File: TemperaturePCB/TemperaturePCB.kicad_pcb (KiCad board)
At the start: 2 copper layers, 16 x 24.8 mm, 3 parts, among them J1 Conn_01x02_Socket

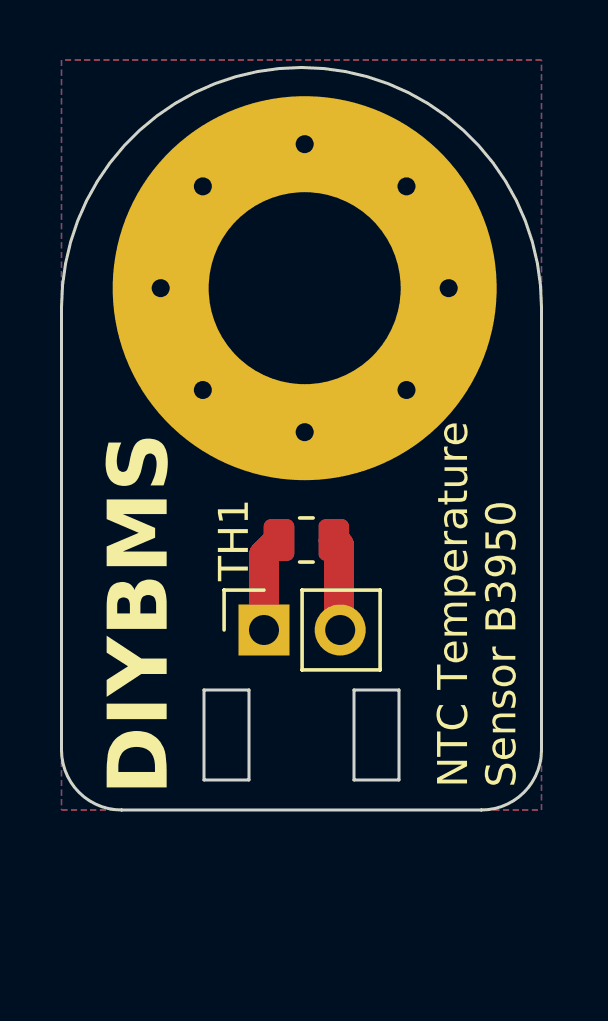
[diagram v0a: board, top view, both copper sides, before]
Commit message: Squashed commit of the following:
commit 382df4b7a104fb34cc4a4da3f786b21ade19fcd5
Author: GitHub Action <action@github.com>
Date:   Fri Apr 18 11:47:05 2025 +0000

    CI: pcb-artifacts-ModuleV490-AllInOne

commit b35cb7a0d3894cf57b33edb037eb829bc9ec5ea4
Author: Stuart Pittaway <1201909+stuartpittaway@users.noreply.github.com>
Date:   Fri Apr 18 12:44:57 2025 +0100

    Minor tweaks

commit ea046b7e5d836263693da1b47c6dfb3dc918925c
Author: Stuart Pittaway <1201909+stuartpittaway@users.noreply.github.com>
Date:   Fri Apr 18 12:44:16 2025 +0100

    PCB Panel of Temp sensors

commit ba929f4700586b6858203bc466c6b18e911d661e
Author: GitHub Action <action@github.com>
Date:   Sun Mar 23 15:29:50 2025 +0000

    CI: pcb-artifacts-ModuleV490-AllInOne

commit 1dbbac7378fdc5acb48c43d3f728917ce2318f16
Author: GitHub Action <action@github.com>
Date:   Wed Apr 10 09:57:21 2024 +0000

    CI: pcb-artifacts-ModuleV490-AllInOne

commit 35f617d42fc7a6a7ab395d232005d3307c26595c
Author: Stuart Pittaway <1201909+stuartpittaway@users.noreply.github.com>
Date:   Wed Apr 10 10:55:49 2024 +0100

    Update pcb-artifacts-modulev490-allinone.yaml

commit c8295c0089ea2c5e86742be6a5572142963deb8f
Author: Stuart Pittaway <1201909+stuartpittaway@users.noreply.github.com>
Date:   Wed Apr 10 10:53:50 2024 +0100

    Update pcb-artifacts-modulev490-allinone.yaml

commit d19b2989a6afd4cac4ecf3c8c78554eedba7b99a
Author: Stuart Pittaway <1201909+stuartpittaway@users.noreply.github.com>
Date:   Wed Apr 10 10:50:28 2024 +0100

    Update pcb-artifacts-modulev490-allinone.yaml

commit 8478886fe70d1ee53aca3bbd908099e6f38ff11d
Author: Stuart Pittaway <1201909+stuartpittaway@users.noreply.github.com>
Date:   Wed Apr 10 10:41:28 2024 +0100

    Update pcb-artifacts-modulev490-allinone.yaml

commit afeafa74721a9b51459c6106f0a15ae423229204
Author: Stuart Pittaway <1201909+stuartpittaway@users.noreply.github.com>
Date:   Wed Apr 10 10:39:10 2024 +0100

    Inductor part change - fix workflows

commit 70fd25ba43b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
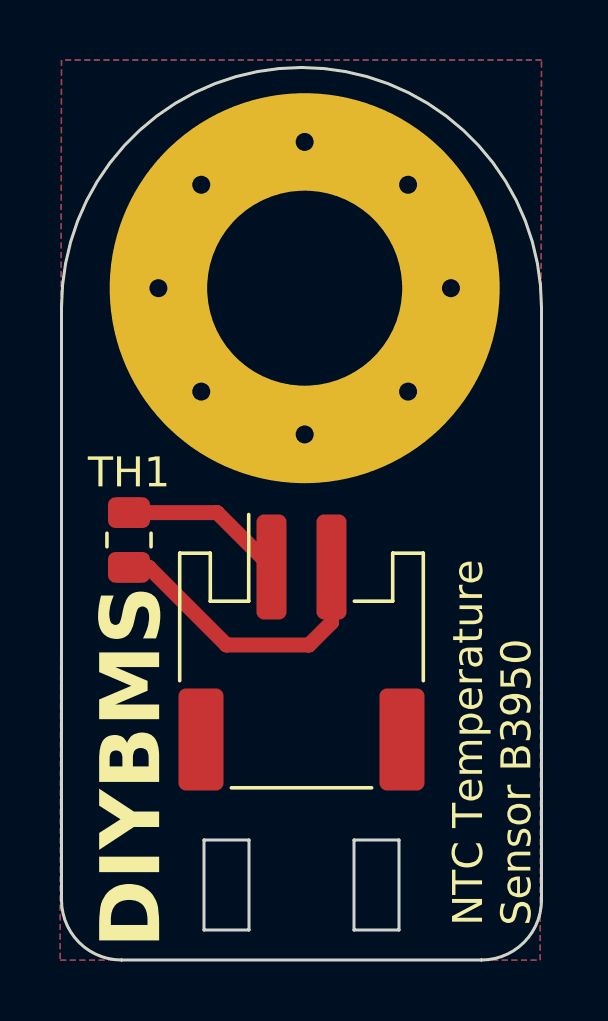
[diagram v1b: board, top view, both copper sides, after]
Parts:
- H1: footprint MountingHole:MountingHole_6.4mm_M6_Pad_Via -> MountingHole:MountingHole_6.5mm_Pad_Via
- J1: value Conn_01x02_Socket -> S2B-PH-SM4-TB(LF)(SN); footprint Connector_PinSocket_2.54mm:PinSocket_1x02_P2.54mm_Vertical -> Connector_JST:JST_PH_S2B-PH-SM4-TB_1x02-1MP_P2.00mm_Horizontal
- moved TH1 5.91 mm to (135.5, 105.0), turned to 90 degrees
- moved J1 1.46 mm to (141.2, 108.8), turned to 0 degrees
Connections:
- TH1 pad 1: Net-(J1-Pin_1) -> Net-(J1-Pin_2)
- TH1 pad 2: Net-(J1-Pin_2) -> Net-(J1-Pin_1)
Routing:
- net Net-(J1-Pin_2): track 3.09 -> 9.98 mm
- net Net-(J1-Pin_1): track 3.21 -> 5.50 mm
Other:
- board size 16 x 24.8 mm -> 16 x 29.8 mm
